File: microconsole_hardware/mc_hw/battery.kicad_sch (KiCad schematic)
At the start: 19 parts, among them J1 USB_C_Receptacle_USB2.0_16P, Q1 Q_PMOS_GSD, SW1 SW_Nidec_CAS-120A1, U1 MCP73833_MSOP, U2 S2B-PH-K-S

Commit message: fix up everything,
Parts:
- Q1: footprint (none) -> Package_TO_SOT_THT:TO-92
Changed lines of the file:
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@@
 		)
 		(instances
-			(project "mc_hw"
+			(project "top"
 				(path "/3433afdc-e53a-48bd-a2b1-9fdee73e8b40/2e88eeda-748f-4d75-b88b-5acda3278369"
 					(reference "R6")
@@
 		)
 		(instances
-			(project "mc_hw"
+			(project "top"
 				(path "/3433afdc-e53a-48bd-a2b1-9fdee73e8b40/2e88eeda-748f-4d75-b88b-5acda3278369"
 					(reference "R5")
@@
 		)
 		(instances
-			(project "mc_hw"
+			(project "top"
 				(path "/3433afdc-e53a-48bd-a2b1-9fdee73e8b40/2e88eeda-748f-4d75-b88b-5acda3278369"
 					(reference "R7")
@@
 		)
 		(instances
-			(project "mc_hw"
+			(project "top"
 				(path "/3433afdc-e53a-48bd-a2b1-9fdee73e8b40/2e88eeda-748f-4d75-b88b-5acda3278369"
 					(reference "C1")
@@
 		)
 		(instances
-			(project "mc_hw"
+			(project "top"
 				(path "/3433afdc-e53a-48bd-a2b1-9fdee73e8b40/2e88eeda-748f-4d75-b88b-5acda3278369"
 					(reference "U1")
@@
 		)
 		(instances
-			(project "mc_hw"
+			(project "top"
 				(path "/3433afdc-e53a-48bd-a2b1-9fdee73e8b40/2e88eeda-748f-4d75-b88b-5acda3278369"
 					(reference "J1")
@@
 		)
 		(instances
-			(project "mc_hw"
+			(project "top"
 				(path "/3433afdc-e53a-48bd-a2b1-9fdee73e8b40/2e88eeda-748f-4d75-b88b-5acda3278369"
 					(reference "U2")
@@
 		)
 		(instances
-			(project "mc_hw"
+			(project "top"
 				(path "/3433afdc-e53a-48bd-a2b1-9fdee73e8b40/2e88eeda-748f-4d75-b88b-5acda3278369"
 					(reference "D1")
@@
 		)
 		(instances
-			(project "mc_hw"
+			(project "top"
 				(path "/3433afdc-e53a-48bd-a2b1-9fdee73e8b40/2e88eeda-748f-4d75-b88b-5acda3278369"
 					(reference "R9")
@@
 			)
 		)
-		(property "Footprint" ""
+		(property "Footprint" "Package_TO_SOT_THT:TO-92"
 			(at 123.19 60.96 0)
 			(hide yes)
@@
 		)
 		(instances
-			(project "mc_hw"
+			(project "top"
 				(path "/3433afdc-e53a-48bd-a2b1-9fdee73e8b40/2e88eeda-748f-4d75-b88b-5acda3278369"
 					(reference "Q1")
@@
 		)
 		(instances
-			(project "mc_hw"
+			(project "top"
 				(path "/3433afdc-e53a-48bd-a2b1-9fdee73e8b40/2e88eeda-748f-4d75-b88b-5acda3278369"
 					(reference "SW1")
@@
 		)
 		(instances
-			(project "mc_hw"
+			(project "top"
 				(path "/3433afdc-e53a-48bd-a2b1-9fdee73e8b40/2e88eeda-748f-4d75-b88b-5acda3278369"
 					(reference "D4")
@@
 		)
 		(instances
-			(project "mc_hw"
+			(project "top"
 				(path "/3433afdc-e53a-48bd-a2b1-9fdee73e8b40/2e88eeda-748f-4d75-b88b-5acda3278369"
 					(reference "R8")
@@
 		)
 		(instances
-			(project "mc_hw"
+			(project "top"
 				(path "/3433afdc-e53a-48bd-a2b1-9fdee73e8b40/2e88eeda-748f-4d75-b88b-5acda3278369"
 					(reference "R10")
@@
 		)
 		(instances
-			(project "mc_hw"
+			(project "top"
 				(path "/3433afdc-e53a-48bd-a2b1-9fdee73e8b40/2e88eeda-748f-4d75-b88b-5acda3278369"
 					(reference "C2")
@@
 		)
 		(instances
-			(project "mc_hw"
+			(project "top"
 				(path "/3433afdc-e53a-48bd-a2b1-9fdee73e8b40/2e88eeda-748f-4d75-b88b-5acda3278369"
 					(reference "D2")
@@
 		)
 		(instances
-			(project "mc_hw"
+			(project "top"
 				(path "/3433afdc-e53a-48bd-a2b1-9fdee73e8b40/2e88eeda-748f-4d75-b88b-5acda3278369"
 					(reference "D3")
@@
 		)
 		(instances
-			(project "mc_hw"
+			(project "top"
 				(path "/3433afdc-e53a-48bd-a2b1-9fdee73e8b40/2e88eeda-748f-4d75-b88b-5acda3278369"
 					(reference "R3")
@@
 		)
 		(instances
-			(project "mc_hw"
+			(project "top"
 				(path "/3433afdc-e53a-48bd-a2b1-9fdee73e8b40/2e88eeda-748f-4d75-b88b-5acda3278369"
 					(reference "R4")

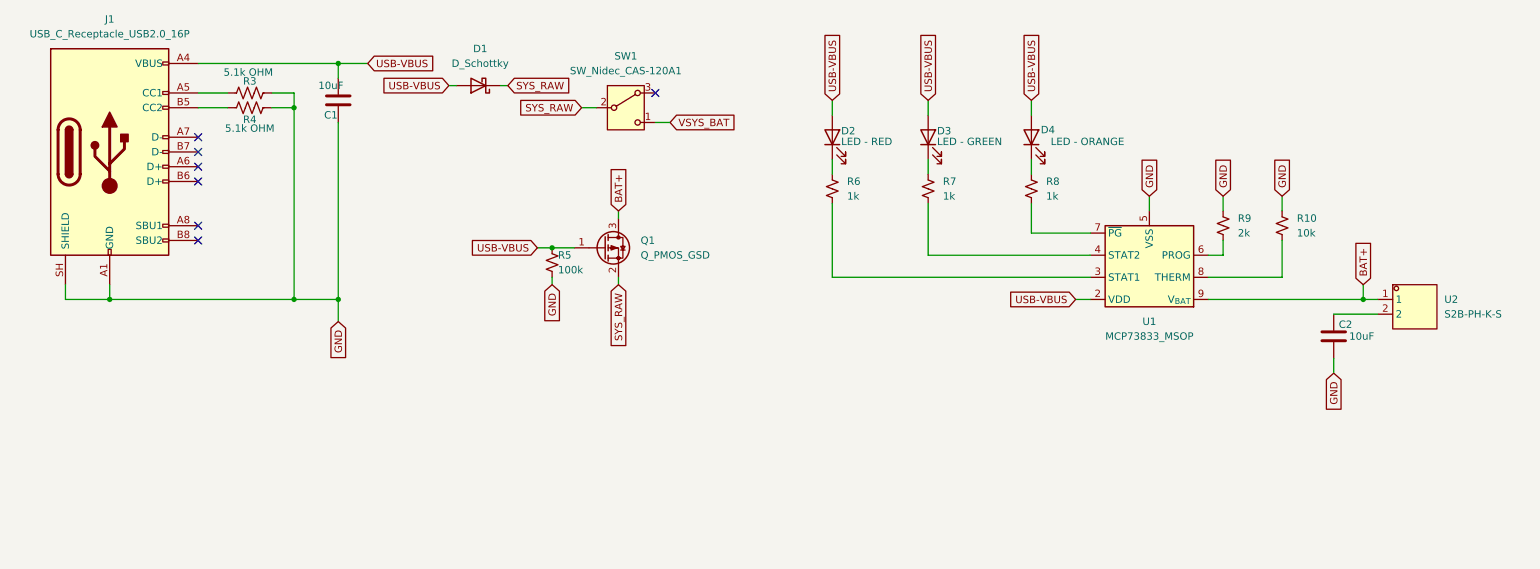
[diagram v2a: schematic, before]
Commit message: fix up design and parts
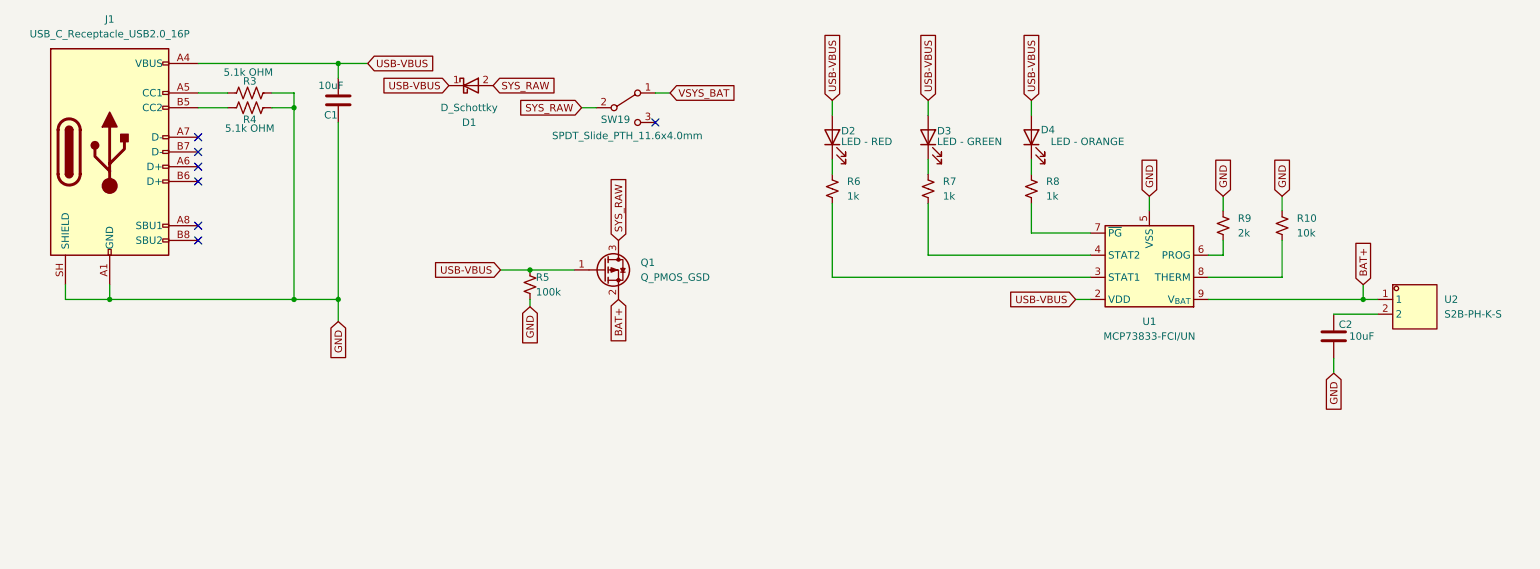
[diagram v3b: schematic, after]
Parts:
- removed SW1: SW_Nidec_CAS-120A1, Button_Switch_SMD:Nidec_Copal_CAS-120A, symbol Switch:SW_Nidec_CAS-120A1
- added SW19: SPDT_Slide_PTH_11.6x4.0mm, PCM_SparkFun-Switch:Slide_SPDT_PTH_11.6x4.0mm, symbol PCM_SparkFun-Switch:SPDT_Slide_PTH_11.6x4.0mm
- D1: footprint PCM_SparkFun-Sensor:Sensirion_DFN-4_1.5x1.5mm_P0.8mm_SHT4x_NoCentralPad -> Diode_SMD:Nexperia_CFP3_SOD-123W
- J1: symbol Connector:USB_C_Receptacle_USB2.0_16P -> project_parts:USB_C_Receptacle_USB2.0_16P
- Q1: footprint Package_TO_SOT_THT:TO-92 -> Package_TO_SOT_SMD:SOT-23
- U1: value MCP73833_MSOP -> MCP73833-FCI/UN
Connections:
- net BAT+: now also Q1.2 (S); no longer Q1.3 (D)
- net SYS_RAW: now also D1.2 (A), Q1.3 (D), SW19.2 (B); no longer D1.1 (K), Q1.2 (S)
- net VDD: now also D1.1 (K); no longer D1.2 (A)
- net VSYS_BAT: now also SW19.1 (A)
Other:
- moved on the sheet: R5

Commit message: fix up power and parts
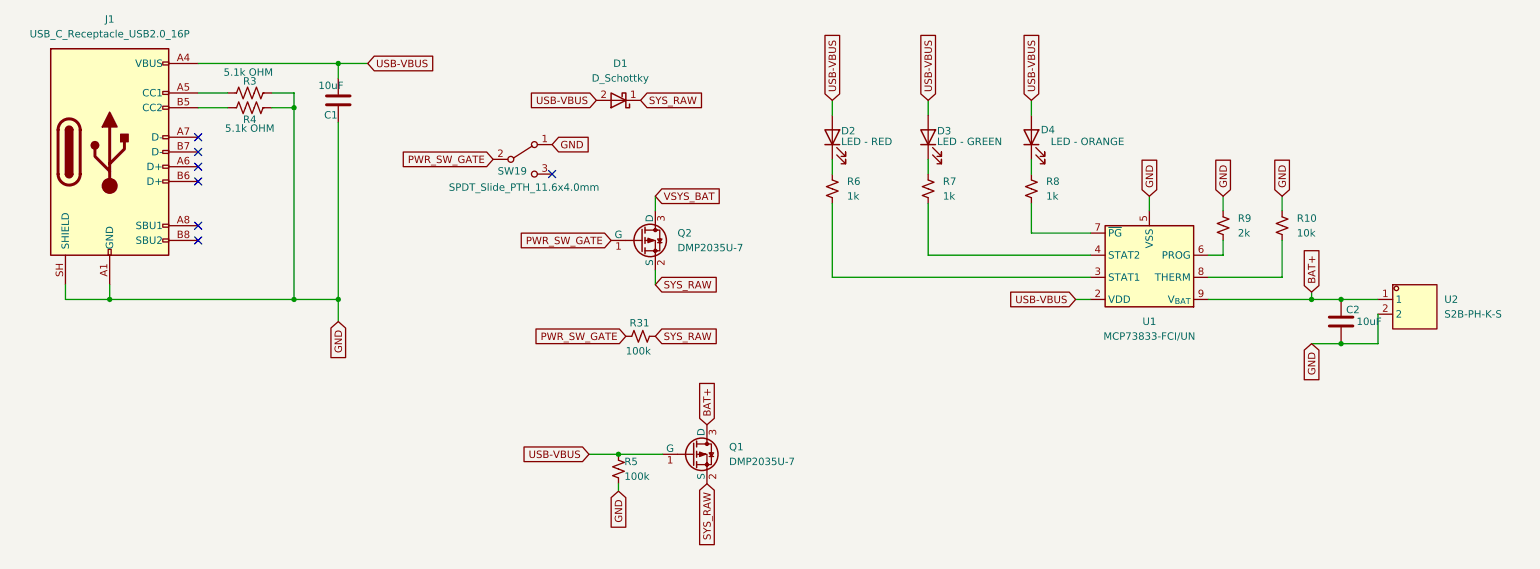
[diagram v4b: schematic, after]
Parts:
- added Q2: DMP2035U-7, Package_TO_SOT_SMD:SOT-23, symbol Transistor_FET:Q_PMOS_GSD
- added R31: 100k, PCM_SparkFun-Resistor:R_0603_1608Metric, symbol PCM_SparkFun-Resistor:0.47_0603
- Q1: value Q_PMOS_GSD -> DMP2035U-7
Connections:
- net BAT+: now also C2.1, Q1.3 (D); no longer Q1.2 (S)
- net GND: now also SW19.1 (A), U2.2
- net SYS_RAW: now also D1.1 (K), Q1.2 (S), Q2.2 (S), R31.1; no longer D1.2 (A), Q1.3 (D), SW19.2 (B)
- net VDD: now also D1.2 (A); no longer D1.1 (K)
- net VSYS_BAT: now also Q2.3 (D); no longer SW19.1 (A)
- new net PWR_SW_GATE: Q2.1 (G), R31.2, SW19.2 (B)
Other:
- moved on the sheet: D1, R5, SW19
